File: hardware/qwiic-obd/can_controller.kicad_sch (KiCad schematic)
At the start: 7 parts, among them U801 SC18IS602BIPW_128, U802 MCP2515-xST, X801 ASV-12.000MHZ-EJ-T

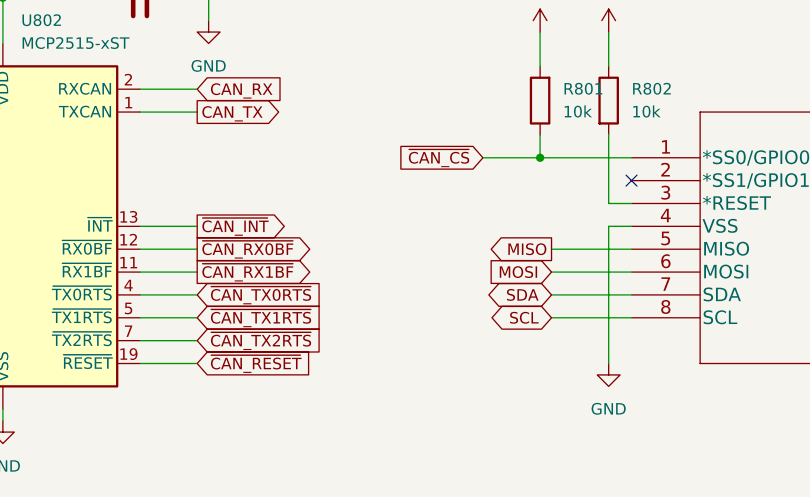
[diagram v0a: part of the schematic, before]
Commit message: Added initial layout (parts dump)
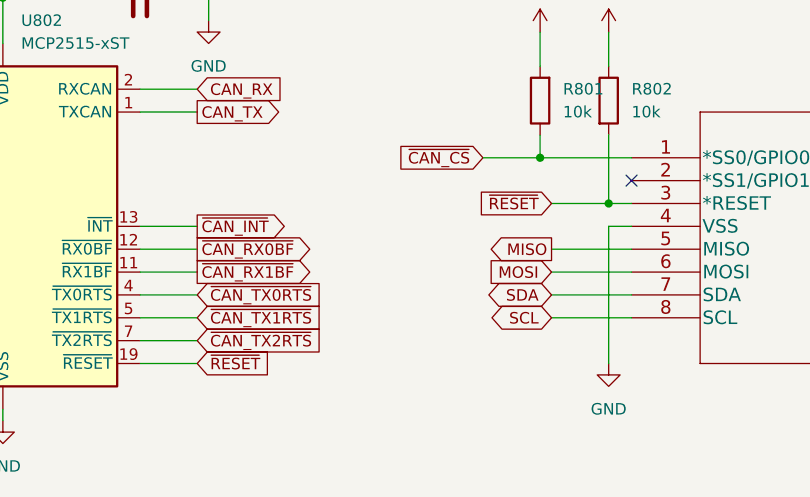
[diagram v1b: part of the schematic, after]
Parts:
- R801, R802, R803: footprint (none) -> Resistor_SMD:R_0805_2012Metric_Pad1.20x1.40mm_HandSolder
- U801: footprint TSSOP16_SOT403-1_NXP -> UltraLibrarian:SC18IS602BIPW_128
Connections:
- net ~{CAN_RESET} is gone; now on net ~{RESET}: U802.19 (~{RESET})
- net ~{RESET}: now reaches R802.2, U801.3 (*RESET)
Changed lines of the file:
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@@
   (junction (at 259.08 86.36) (diameter 0) (color 0 0 0 0)
+  )
+  (junction (at 182.88 86.36) (diameter 0) (color 0 0 0 0)
   )
   (junction (at 264.16 99.06) (diameter 0) (color 0 0 0 0)
@@
     (stroke (width 0) (type default) (color 0 0 0 0))
   )
+  (wire (pts (xy 176.53 86.36) (xy 182.88 86.36))
+    (stroke (width 0) (type default) (color 0 0 0 0))
+  )
   (wire (pts (xy 130.81 96.52) (xy 137.16 96.52))
     (stroke (width 0) (type default) (color 0 0 0 0))
@@
     )
   )
+  (global_label "~{RESET}" (shape input) (at 176.53 86.36 180) (fields_autoplaced)
+    (effects (font (size 1.27 1.27)) (justify right))
+    (property "Intersheet References" "${INTERSHEET_REFS}" (id 0) (at 168.3717 86.2806 0)
+      (effects (font (size 1.27 1.27)) (justify right) hide)
+    )
+  )
   (global_label "~{CAN_CS}" (shape input) (at 91.44 78.74 180) (fields_autoplaced)
     (effects (font (size 1.27 1.27)) (justify right))
@@
     )
   )
-  (global_label "~{CAN_RESET}" (shape input) (at 137.16 104.14 0) (fields_autoplaced)
-    (effects (font (size 1.27 1.27)) (justify left))
-    (property "Intersheet References" "${INTERSHEET_REFS}" (id 0) (at 149.975 104.0606 0)
+  (global_label "~{RESET}" (shape input) (at 137.16 104.14 0) (fields_autoplaced)
+    (effects (font (size 1.27 1.27)) (justify left))
+    (property "Intersheet References" "${INTERSHEET_REFS}" (id 0) (at 145.3183 104.0606 0)
       (effects (font (size 1.27 1.27)) (justify left) hide)
     )
@@
       (effects (font (size 1.27 1.27)) (justify left))
     )
-    (property "Footprint" "" (id 2) (at 262.382 77.47 90)
+    (property "Footprint" "Resistor_SMD:R_0805_2012Metric_Pad1.20x1.40mm_HandSolder" (id 2) (at 262.382 77.47 90)
       (effects (font (size 1.27 1.27)) hide)
     )
@@
       (effects (font (size 1.27 1.27)) (justify right))
     )
-    (property "Footprint" "" (id 2) (at 177.038 74.93 90)
+    (property "Footprint" "Resistor_SMD:R_0805_2012Metric_Pad1.20x1.40mm_HandSolder" (id 2) (at 177.038 74.93 90)
       (effects (font (size 1.27 1.27)) hide)
     )
@@
       (effects (font (size 1.524 1.524)))
     )
-    (property "Footprint" "TSSOP16_SOT403-1_NXP" (id 2) (at 218.44 75.184 0)
+    (property "Footprint" "UltraLibrarian:SC18IS602BIPW_128" (id 2) (at 218.44 75.184 0)
       (effects (font (size 1.524 1.524)) hide)
     )
@@
       (effects (font (size 1.27 1.27)) (justify left))
     )
-    (property "Footprint" "" (id 2) (at 181.102 74.93 90)
-      (effects (font (size 1.27 1.27)) hide)
-    )
+    (property "Footprint" "Resistor_SMD:R_0805_2012Metric_Pad1.20x1.40mm_HandSolder" (id 2) (at 181.102 74.93 90)
+      (effects (font (size 1.27 1.27)) hide)
+    )
